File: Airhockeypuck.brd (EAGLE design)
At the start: 60 x 60 mm, 23 parts, among them J1 USB-MB-H

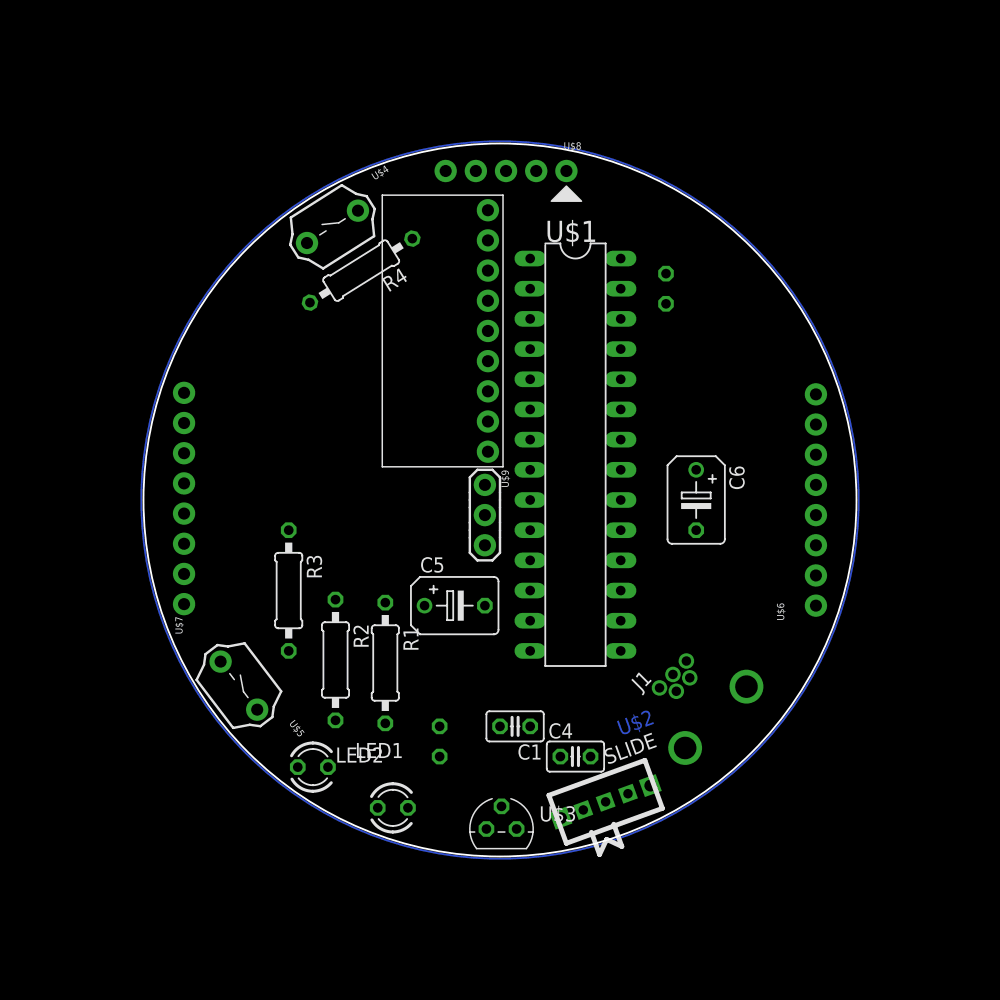
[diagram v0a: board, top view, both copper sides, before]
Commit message: minor edits
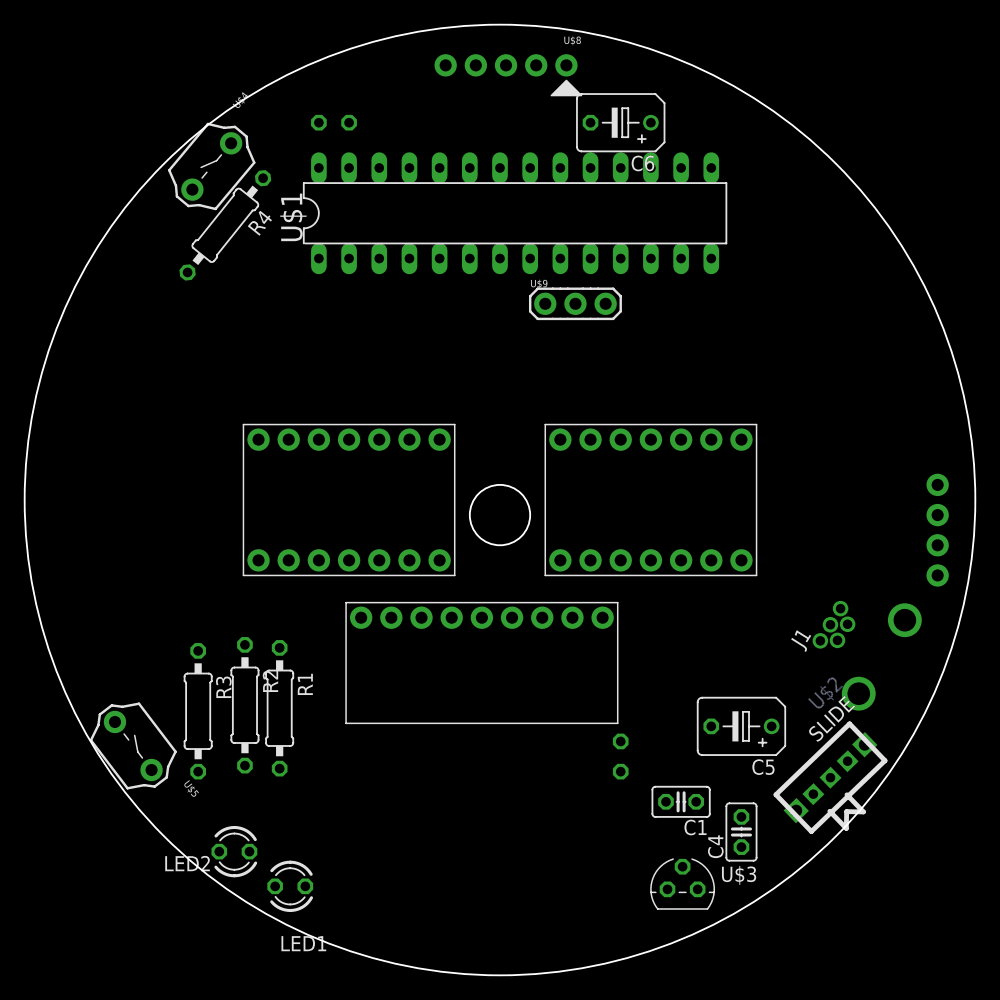
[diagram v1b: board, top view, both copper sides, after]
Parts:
- added U$11: HC-08, MEE_433:HC-08
- U$6, U$7: value CONN_08 -> DRV8835; device MEE_433:1X08 -> MEE_433:DRV8835
- moved U$6 40.3 mm to (-12.7, 1.27)
- moved U$7 40.3 mm to (12.7, 1.27), turned to 270 degrees
- moved C6 32.4 mm to (10.2, 33.0), turned to 180 degrees
- moved C3 31.2 mm to (-14.0, 33.0), turned to 180 degrees
- moved C5 26.2 mm to (20.3, -17.8), turned to 180 degrees
- moved U$1 20.9 mm to (1.27, 25.4), turned to 0 degrees
- moved U$9 19.3 mm to (6.35, 17.8), turned to 0 degrees
- moved U$2 19.0 mm to (27.8, -22.1), turned to 223.9 degrees
- moved U$10 17.0 mm to (8.64, -8.64), turned to 180 degrees
- moved U$3 16.1 mm to (15.4, -31.5)
- moved C1 15.3 mm to (15.2, -24.1)
- moved C4 15.3 mm to (20.3, -26.7), turned to 90 degrees
- moved C2 15.3 mm to (10.2, -20.3), turned to 270 degrees
- moved J1 14.9 mm to (32.1, -11.9), turned to 147.9 degrees
- moved R3 12.7 mm to (-25.4, -16.5)
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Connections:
- new net N$10: U$6.10.BENABLE
- new net N$11: U$6.11.BPHASE
- new net N$12: U$6.12.AENABLE
- new net N$13: U$6.13.APHASE
- new net N$14: U$11.4.RX
- new net N$16: U$7.10.BENABLE
- new net N$17: U$7.11.BPHASE
- new net N$18: U$7.12.AENABLE
- new net N$19: U$7.13.APHASE
- new net N$3: U$11.1.VCC
- new net N$9: U$11.3.TX
- net +3V3: now also U$6.9.VCC, U$7.9.VCC; no longer U$7.2
- net +5V: now also U$2.1.+5V; no longer U$2.1, U$6.2
- net A0: no longer U$7.8
- net A1: no longer U$7.7
- net A4/LED: no longer U$7.3
- net B13: no longer U$6.6
- net B14: no longer U$6.7
- net B15: no longer U$6.8
- net B2: no longer U$7.6
- net B3: no longer U$7.5
- net B4/USER: no longer U$7.4
- net B7: no longer U$6.3
- net B8: no longer U$6.4
- net B9: no longer U$6.5
- net GND: now also U$11.2.GND, U$6.8.GND, U$7.8.GND; no longer U$6.1, U$7.1
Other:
- board size 60 x 60 mm -> 80 x 80 mm
